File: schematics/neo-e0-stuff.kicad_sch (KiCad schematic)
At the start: 4 parts

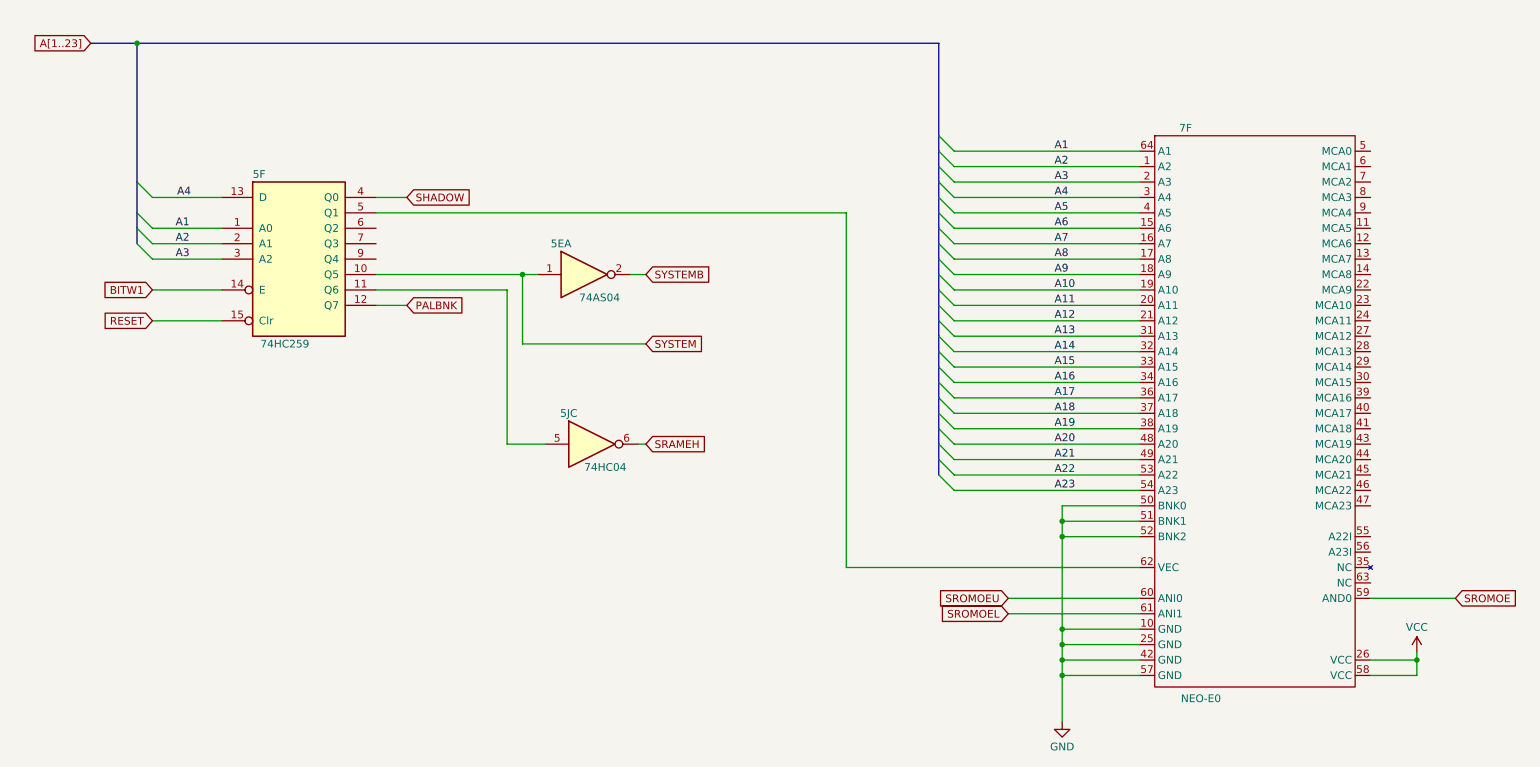
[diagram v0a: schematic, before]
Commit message: WIP
starting Page 2 : LSPC2
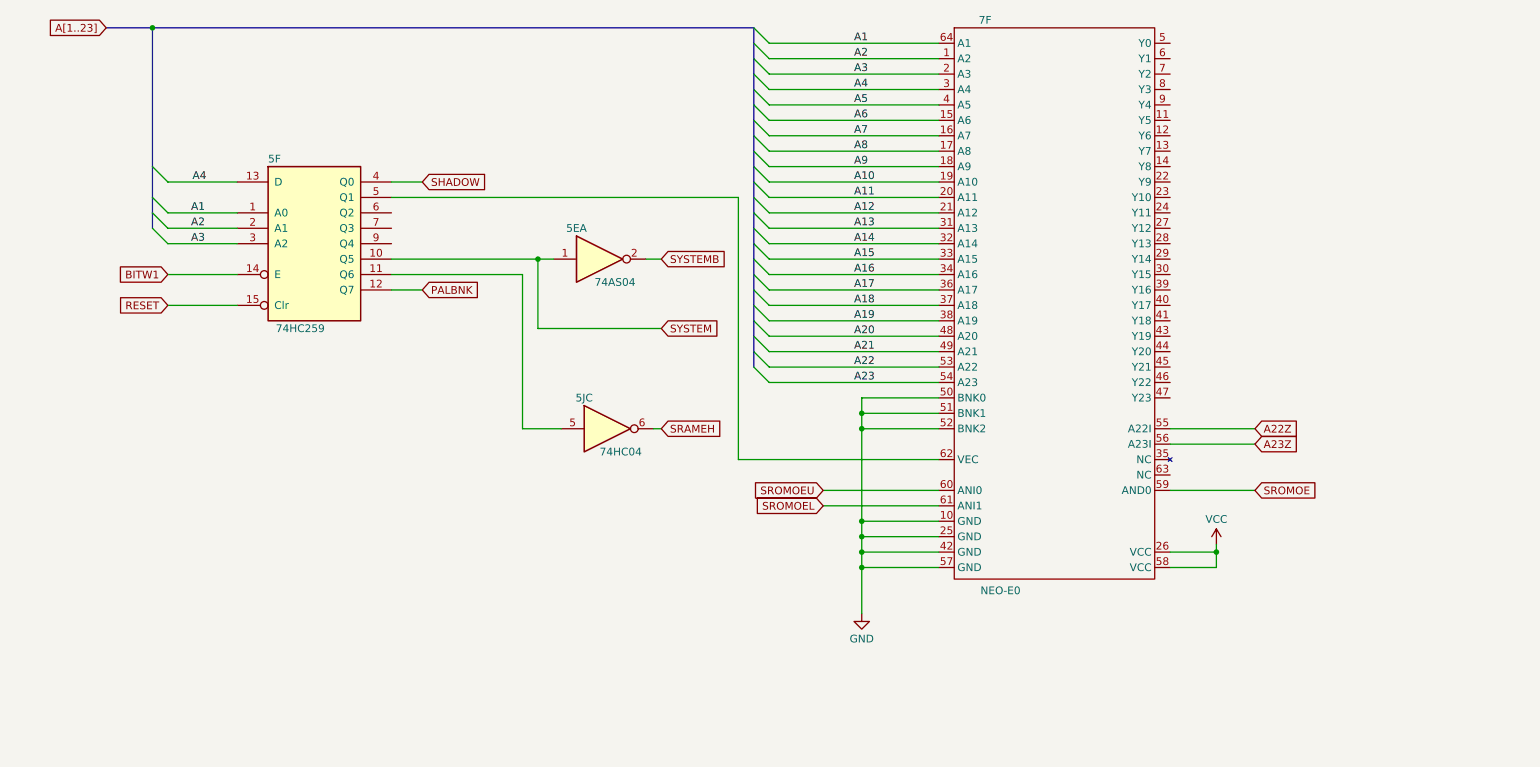
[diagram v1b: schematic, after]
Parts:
- 7F: symbol 0-Custom-SNK:NEO-E0 -> 0-Custom-SNK:NEO-E0 (MV2F)
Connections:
- net A22Z: now reaches 7F.55 (A22I)
- net A23Z: now reaches 7F.56 (A23I)
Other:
- company: (none) -> SNK
- title: (none) -> NEO-EO shift registers
- moved on the sheet: 5EA, 5F, 5JC, 7F
